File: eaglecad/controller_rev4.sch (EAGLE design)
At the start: 91 parts, among them J1 1.27MM-SWD-CONNECTOR, U101 TCAN330, U200 TPS63070, U300 STSPIN230, U301 TSV991ILT, U302 AS5047P, U400 STSPIN250, U401 TSV991ILT, X101 16MHZ-2.5x2mm

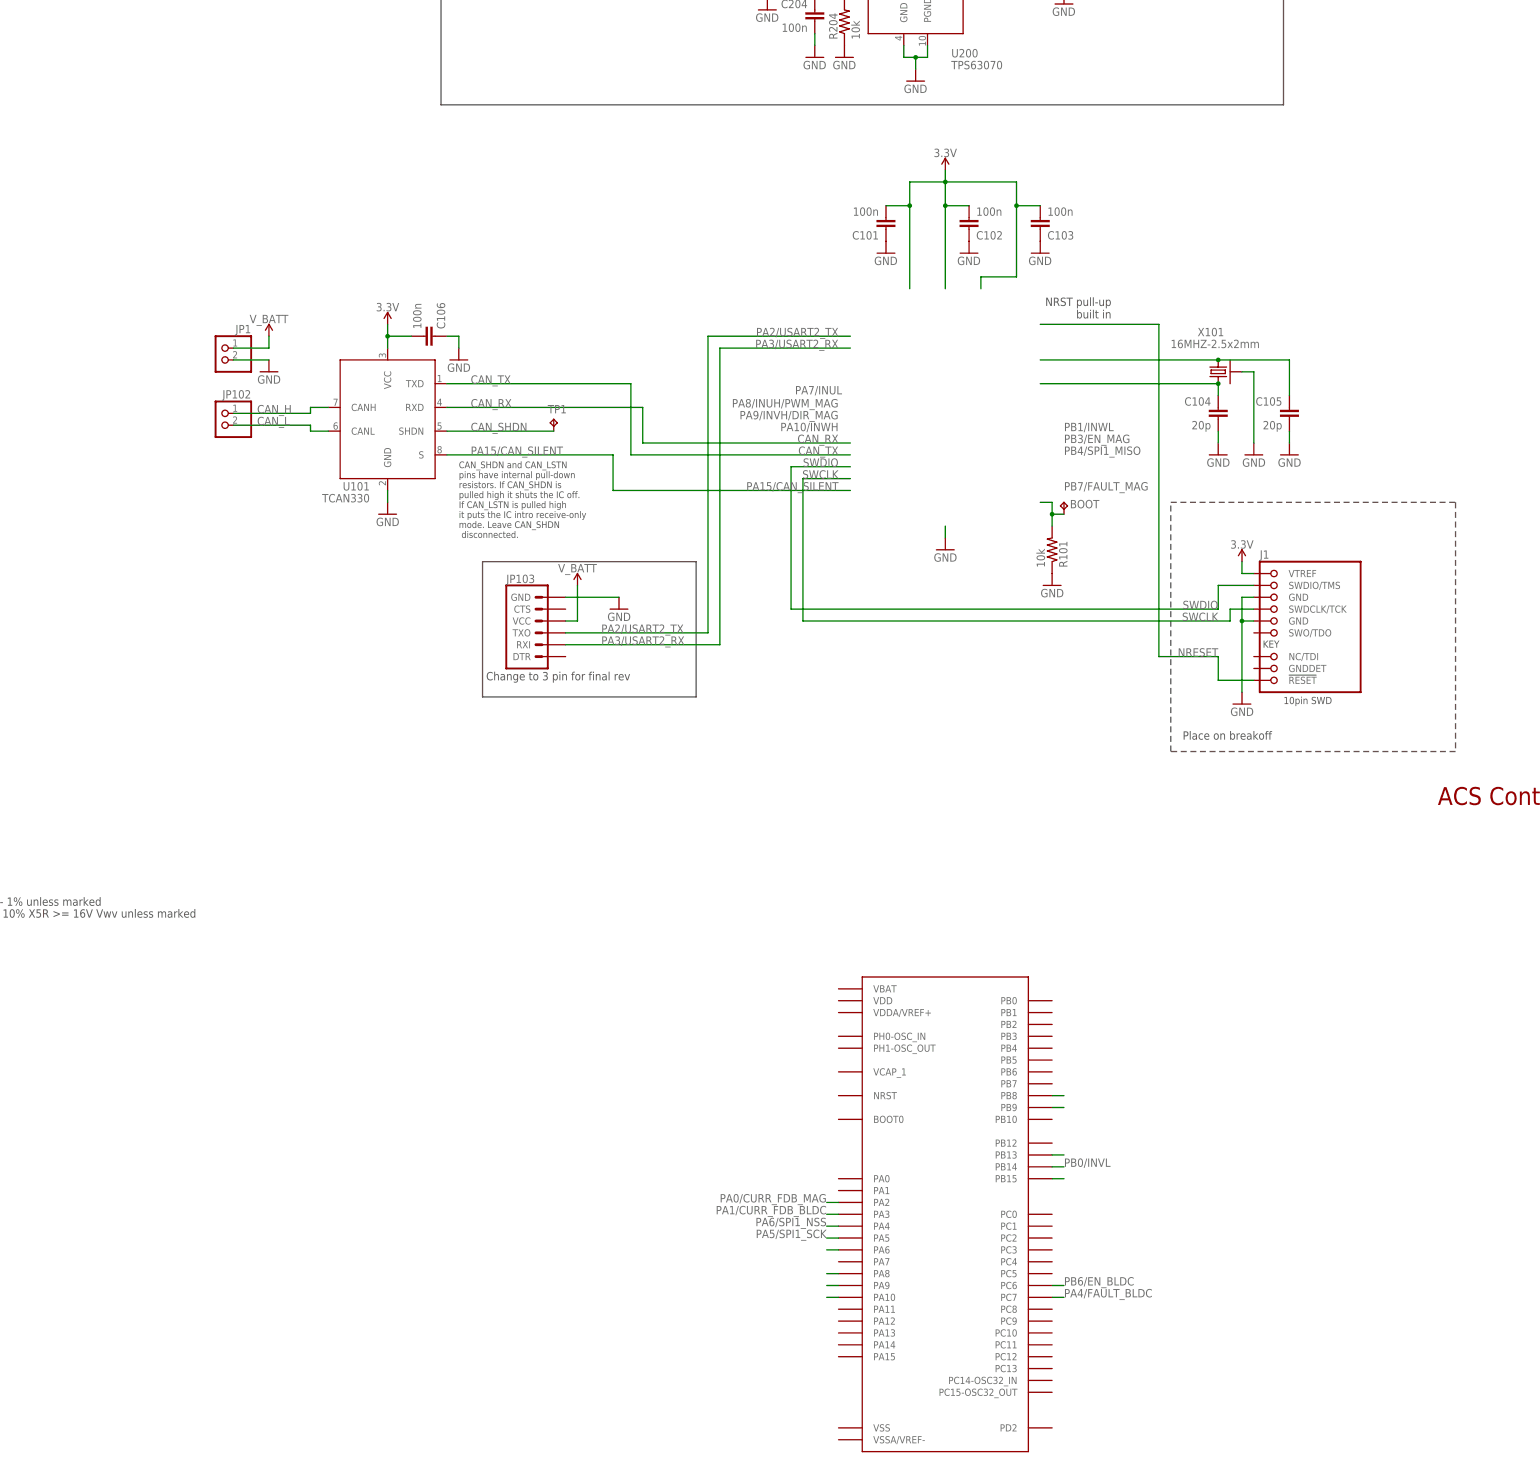
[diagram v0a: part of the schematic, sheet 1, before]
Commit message: f4 updates
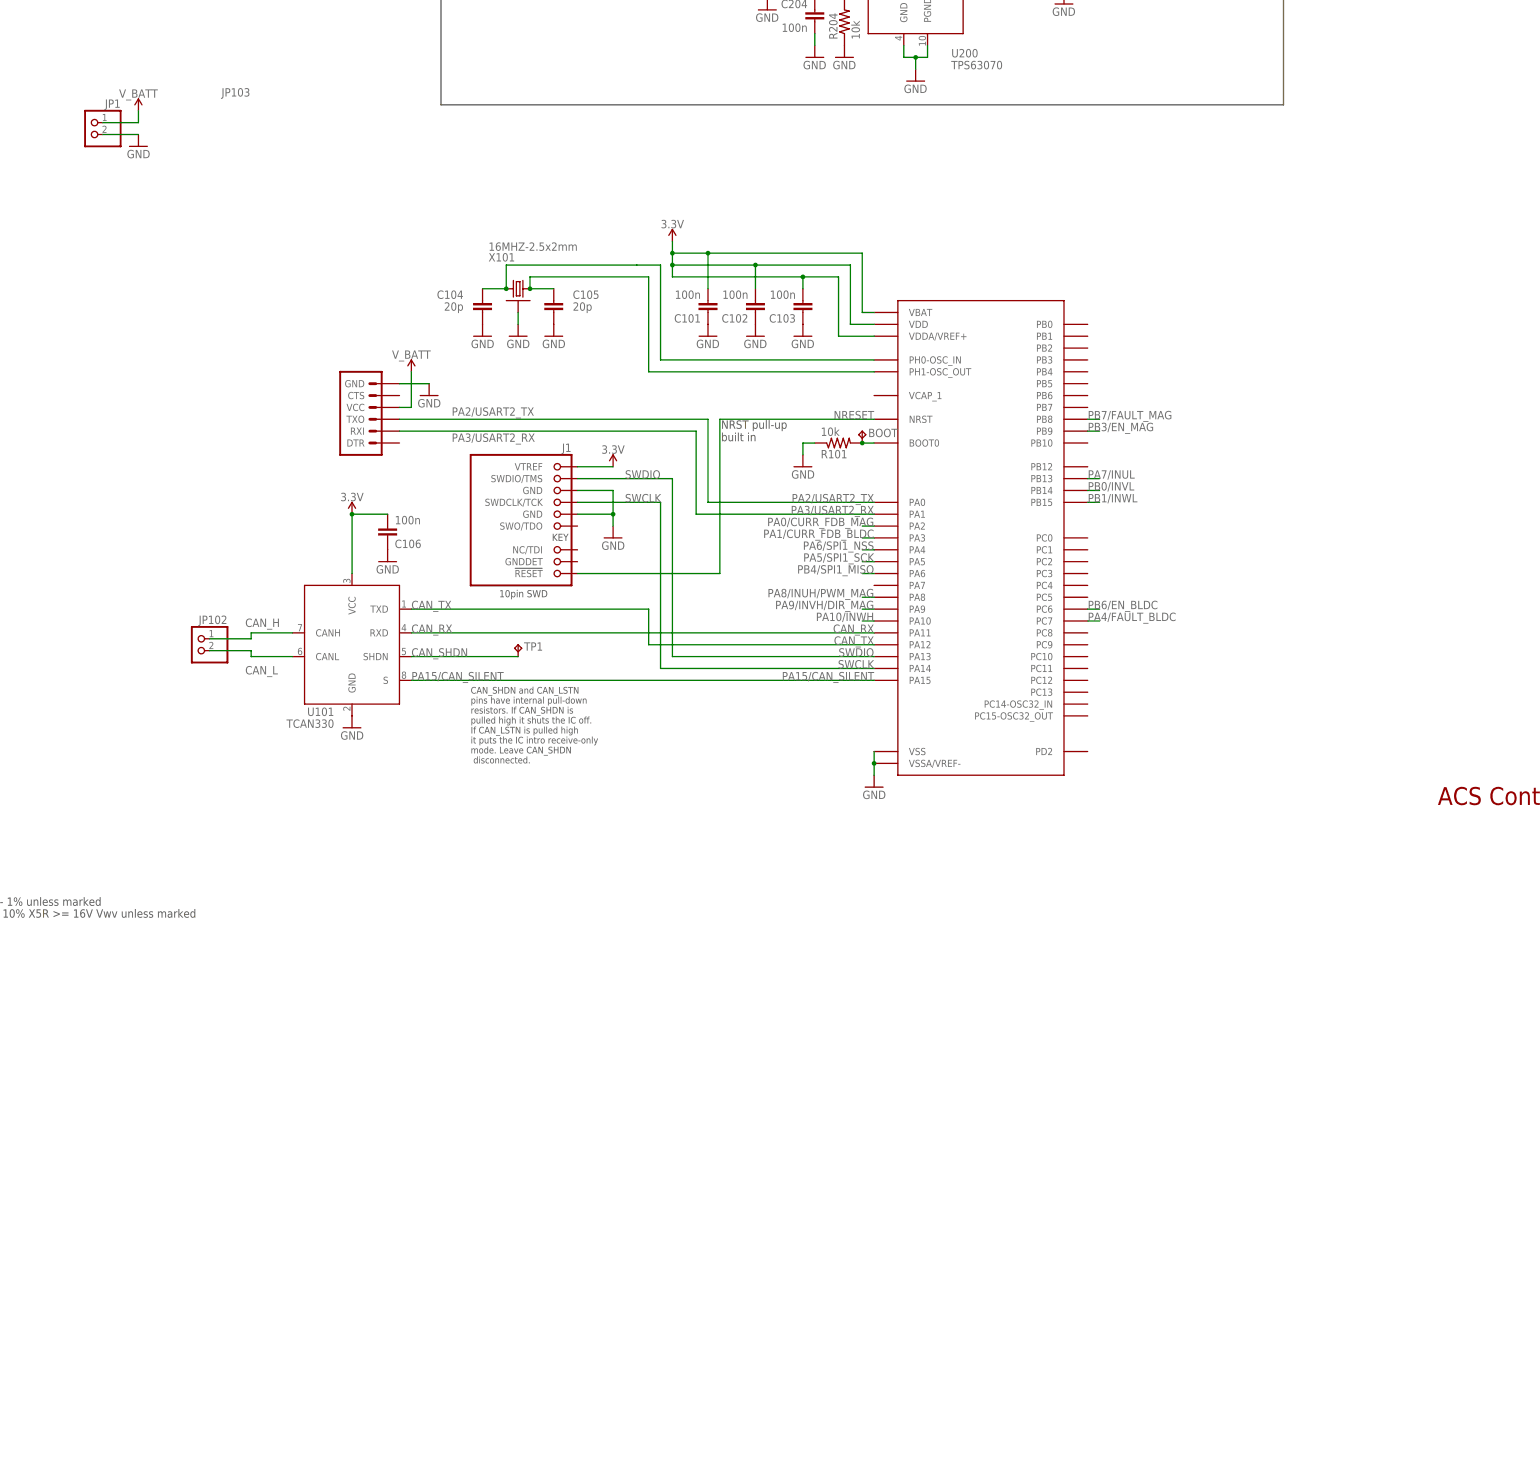
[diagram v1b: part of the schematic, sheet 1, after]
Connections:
- removed net CRYSTALIN: C105.1, X101.1
- removed net CRYSTALOUT: C104.1, X101.2
- new net N$1: C104.2, U$1.PH0-OSC_IN, X101.2
- new net N$4: C105.2, U$1.PH1-OSC_OUT, X101.1
- net 3.3V: now also U$1.VBAT, U$1.VDD, U$1.VDDA/VREF+
- net BOOT: now also U$1.BOOT0
- net CAN_RX: now also U$1.PA11
- net CAN_TX: now also U$1.PA12
- net GND: now also C104.1, C105.1, U$1.VSS, U$1.VSSA/VREF-; no longer C104.2, C105.2
- net NRESET: now also U$1.NRST
- net PA15/CAN_SILENT: now also U$1.PA15
- net PA2/USART2_TX: now also U$1.PA0
- net PA3/USART2_RX: now also U$1.PA1
- net SWCLK: now also U$1.PA14
- net SWDIO: now also U$1.PA13
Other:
- note removed: "Change to 3 pin for final rev"
- note removed: "Place on breakoff"
- moved on the sheet: BOOT, C101, C102, C103, C104, C105, C106, J1, JP1, JP102, JP103, R101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
